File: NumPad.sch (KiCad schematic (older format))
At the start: 73 parts, among them J1 Micro_SD_Card_Det, J2 OLED1, J3 OLED2, J4 Conn_01x05_Female, SW1 SW_SPST, SW10 SW_SPST, SW11 SW_SPST, SW12 SW_SPST, SW13 SW_SPST, SW14 SW_SPST, SW15 SW_SPST, SW16 SW_SPST, SW17 SW_SPST, SW18 SW_SPST, SW19 SW_SPST, SW2 SW_SPST, SW20 SW_SPST, SW21 SW_SPST, SW22 SW_SPST, SW23 SW_SPST, SW24 SW_SPST, SW25 SW_BUTTONRESET, SW26 SW_BUTTON2, SW27 SW_BUTTON1, SW28 SW_BOOT0, SW3 SW_SPST, SW4 SW_SPST, SW5 SW_SPST, SW6 SW_SPST, SW7 SW_SPST, SW8 SW_SPST, SW9 SW_SPST, U1 LM117_TO3, U2 STM32F072C8Tx

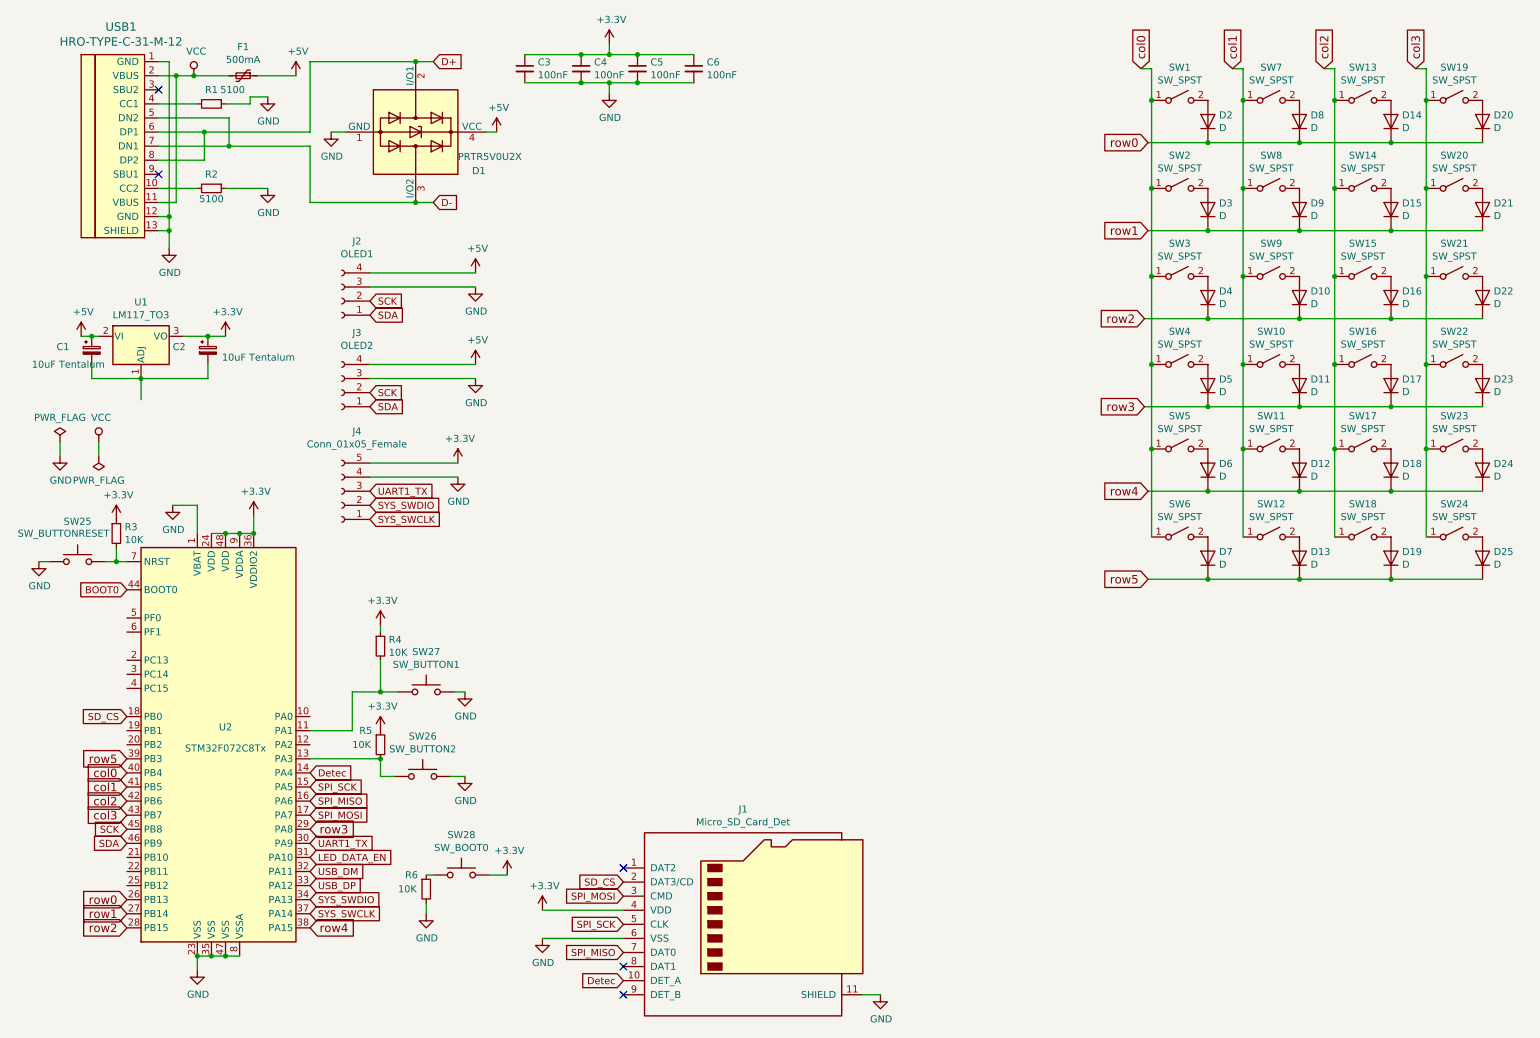
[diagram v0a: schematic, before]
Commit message: Update
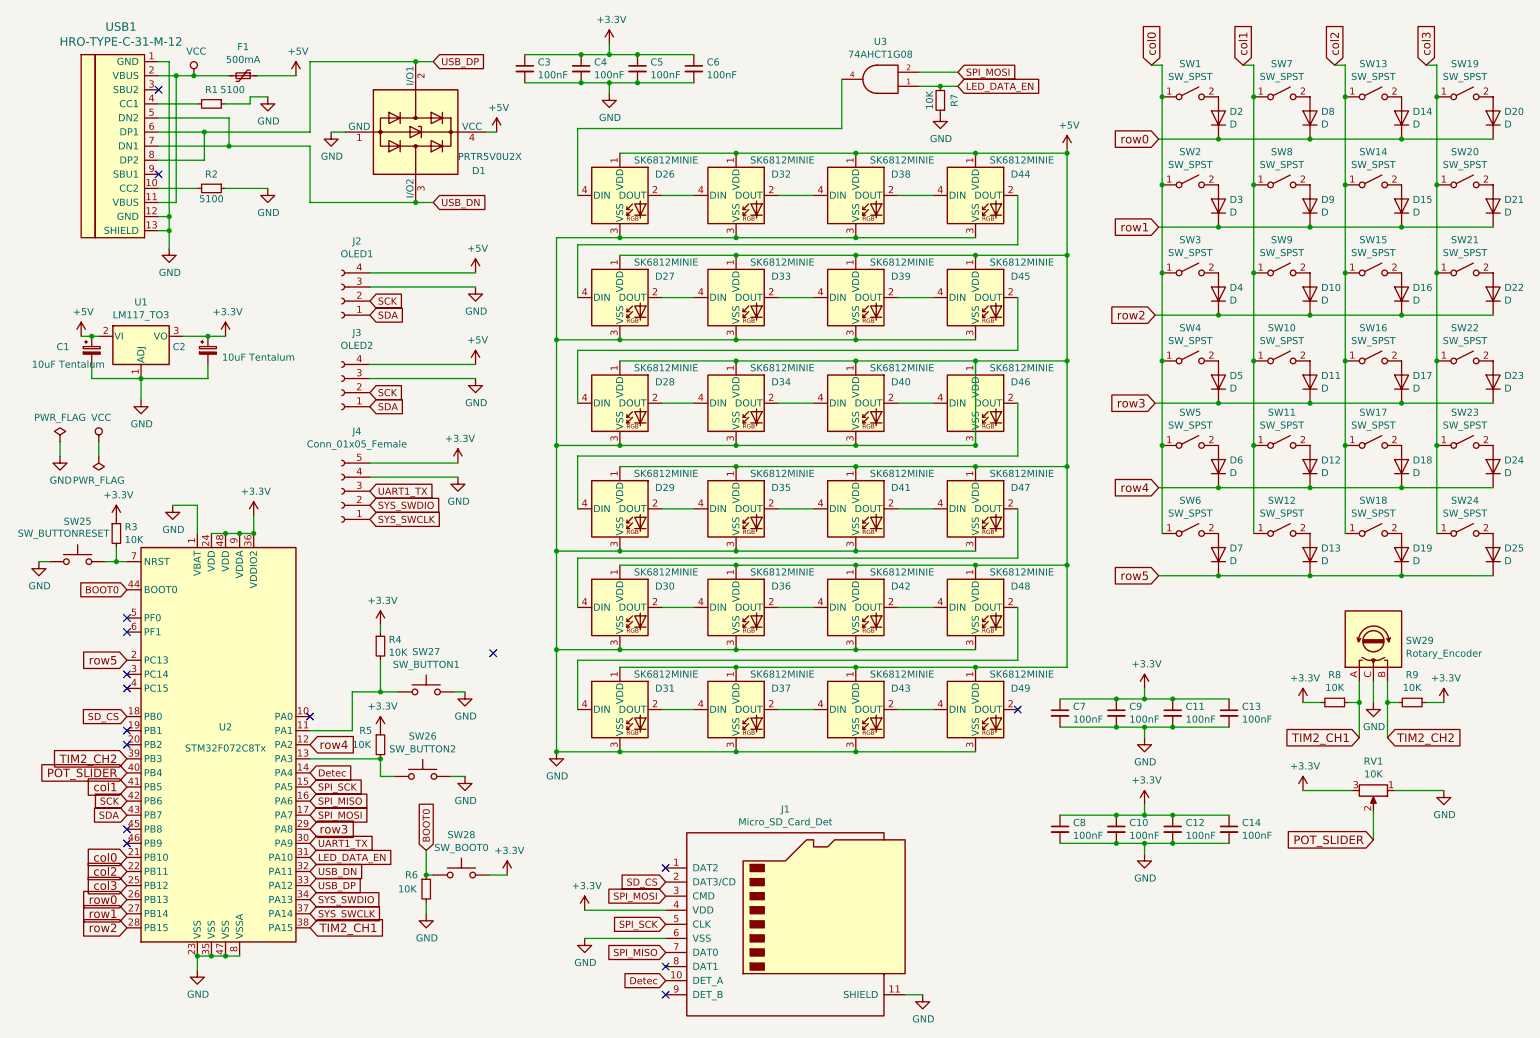
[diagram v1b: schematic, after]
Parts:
- added C10, C11, C12, C13, C14, C7, C8, C9: 100nF, symbol Device:C_Small
- added D26, D27, D28, D29, D30, D31, D32, D33, D34, D35, D36, D37, D38, D39, D40, D41, D42, D43, D44, D45, D46, D47, D48, D49: SK6812MINIE, LED_SMD:LED_SK6812MINI_PLCC4_3.5x3.5mm_P1.75mm, symbol random-keyboard-parts:SK6812MINIE
- added R7, R8, R9: 10K, symbol Device:R_Small
- added RV1: 10K, symbol Device:R_POT
- added SW29: Rotary_Encoder, symbol Device:Rotary_Encoder
- added U3: 74AHCT1G08, symbol 74xGxx:74AHCT1G08
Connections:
- net D+ is gone; now on net USB_DP: D1.2 (I/O1), USB1.6 (DP1), USB1.8 (DP2)
- net GND is gone; now on net +5V: C3.2, C4.2, C5.2, C6.2, D1.1 (GND), J1.11 (SHIELD), J1.6 (VSS), J2.3 (Pin_3), J3.3 (Pin_3), J4.4 (Pin_4), R1.1, R2.1, R6.2, SW25.1, SW26.2, SW27.2, U2.1 (VBAT), U2.23 (VSS), U2.35 (VSS), U2.47 (VSS), U2.8 (VSSA), USB1.1 (GND), USB1.12 (GND), USB1.13 (SHIELD)
- net USB_DM is gone; now on net USB_DN: U2.32 (PA11)
- net +3V3: now also C10.1, C11.1, C12.1, C13.1, C14.1, C7.1, C8.1, C9.1, R8.2, R9.1, RV1.3
- net +5V: now also C1.2, C2.2, U1.1 (ADJ), C10.2, C11.2, C12.2, C13.2, C14.2, C7.2, C8.2, C9.2, D26.1 (VDD), D26.3 (VSS), D27.1 (VDD), D27.3 (VSS), D28.1 (VDD), D28.3 (VSS), D29.1 (VDD), D29.3 (VSS), D30.1 (VDD), D30.3 (VSS), D31.1 (VDD), D31.3 (VSS), D32.1 (VDD), D32.3 (VSS), D33.1 (VDD), D33.3 (VSS), D34.1 (VDD), D34.3 (VSS), D35.1 (VDD), D35.3 (VSS), D36.1 (VDD), D36.3 (VSS), D37.1 (VDD), D37.3 (VSS), D38.1 (VDD), D38.3 (VSS), D39.1 (VDD), D39.3 (VSS), D40.1 (VDD), D40.3 (VSS), D41.1 (VDD), D41.3 (VSS), D42.1 (VDD), D42.3 (VSS), D43.1 (VDD), D43.3 (VSS), D44.1 (VDD), D44.3 (VSS), D45.1 (VDD), D45.3 (VSS), D46.1 (VDD), D46.3 (VSS), D47.1 (VDD), D47.3 (VSS), D48.1 (VDD), D48.3 (VSS), D49.1 (VDD), D49.3 (VSS), R7.1, RV1.1, SW29.C, U3.3 (GND)
- net BOOT0: now also R6.1, SW28.1
- net LED_DATA_EN: now also R7.2, U3.1
- net SCK: now also U2.42 (PB6); no longer U2.45 (PB8)
- net SDA: now also U2.43 (PB7); no longer U2.46 (PB9)
- net SPI_MOSI: now also U3.2
- net VCC: now also U3.5 (VCC)
- net col0: now also U2.21 (PB10); no longer U2.40 (PB4)
- net col2: now also U2.22 (PB11); no longer U2.42 (PB6)
- net col3: now also U2.25 (PB12); no longer U2.43 (PB7)
- net row4: now also U2.12 (PA2); no longer U2.38 (PA15)
- net row5: now also U2.2 (PC13); no longer U2.39 (PB3)
- net D- renamed USB_DN
- new net: D26.2 (DOUT), D32.4 (DIN)
- new net: D26.4 (DIN), U3.4
- new net: D32.2 (DOUT), D38.4 (DIN)
- new net: D38.2 (DOUT), D44.4 (DIN)
- new net: D27.4 (DIN), D44.2 (DOUT)
- new net: D27.2 (DOUT), D33.4 (DIN)
- new net: D33.2 (DOUT), D39.4 (DIN)
- new net: D39.2 (DOUT), D45.4 (DIN)
- new net: D28.4 (DIN), D45.2 (DOUT)
- new net: D28.2 (DOUT), D34.4 (DIN)
- new net: D34.2 (DOUT), D40.4 (DIN)
- new net: D40.2 (DOUT), D46.4 (DIN)
- new net: D29.4 (DIN), D46.2 (DOUT)
- new net: D29.2 (DOUT), D35.4 (DIN)
- new net: D35.2 (DOUT), D41.4 (DIN)
- new net: D41.2 (DOUT), D47.4 (DIN)
- new net: D30.4 (DIN), D47.2 (DOUT)
- new net: D30.2 (DOUT), D36.4 (DIN)
- new net: D36.2 (DOUT), D42.4 (DIN)
- new net: D42.2 (DOUT), D48.4 (DIN)
- new net: D31.4 (DIN), D48.2 (DOUT)
- new net: D31.2 (DOUT), D37.4 (DIN)
- new net: D37.2 (DOUT), D43.4 (DIN)
- new net: D43.2 (DOUT), D49.4 (DIN)
- new net POT_SLIDER: RV1.2, U2.40 (PB4)
- new net TIM2_CH1: R8.1, SW29.A, U2.38 (PA15)
- new net TIM2_CH2: R9.2, SW29.B, U2.39 (PB3)
- no-connect marks 5 -> 16
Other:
- moved on the sheet: D10, D11, D12, D13, D14, D15, D16, D17, D18, D19, D2, D20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
